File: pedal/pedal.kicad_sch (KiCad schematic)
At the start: 55 parts, among them J1 AudioJack3, J2 AudioJack3, J3 Micro SD, J4 USB_B_Micro, J5 Debug, U1 LP2985-1.8, U2 PCM3060, U3 TPS62172DSG, U4 TL072, U5 STM32H750IBTx, U6 RC4580, Y1 25MHz

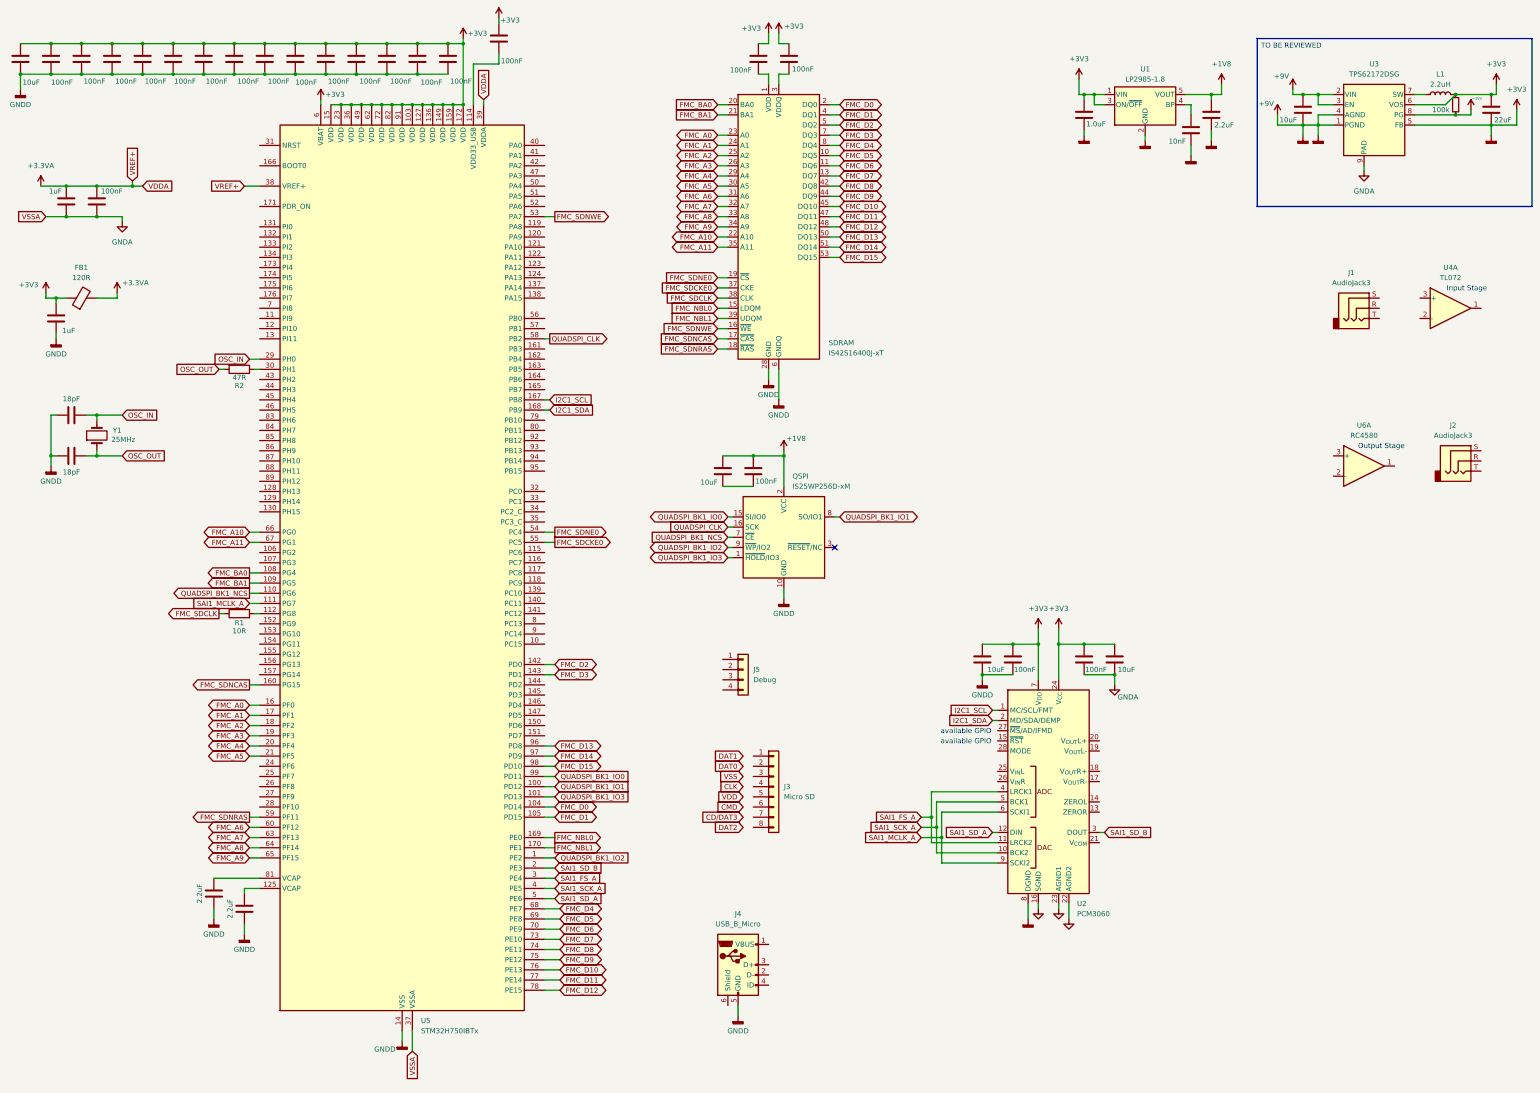
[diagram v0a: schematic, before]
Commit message: update JOURNAL and step down BC
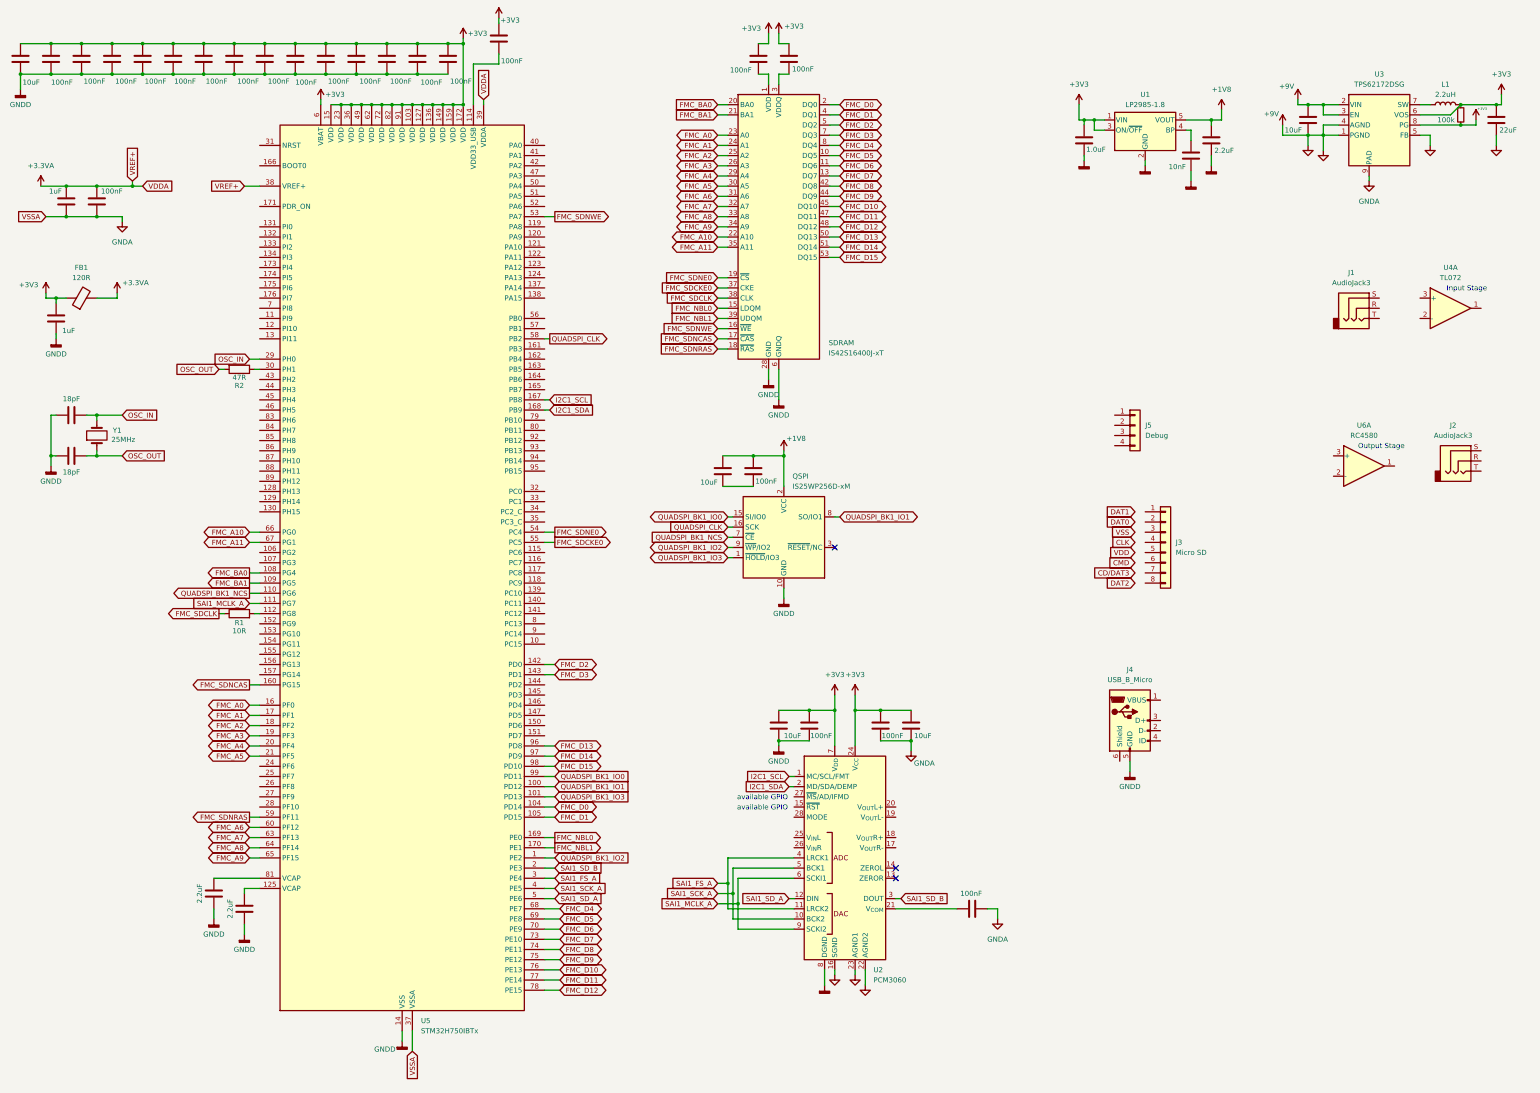
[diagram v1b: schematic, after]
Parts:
- added C37: 100nF, symbol Device:C
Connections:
- net +3V3: no longer C1.1, C10.2, C11.2, C12.2, C13.2, C14.2, C15.2, C16.2, C17.2, C2.1, C21.2, C24.1, C25.1, C26.2, C27.2, C28.2, C29.2, C3.2, C30.1, C30.2, C33.2, C34.2, C4.2, C5.2, C6.2, C7.2, C8.2, C9.2, J4.5 (GND), QSPI.10 (GND), SDRAM.12 (GNDQ), SDRAM.28 (GND), SDRAM.41 (GND), SDRAM.46 (GNDQ), SDRAM.52 (GNDQ), SDRAM.54 (GND), SDRAM.6 (GNDQ), U1.2 (GND), U2.8 (DGND), U3.1 (PGND), U3.2 (VIN), U3.3 (EN), U3.4 (AGND), U3.5 (FB), U5.102 (VSS), U5.113 (VSS), U5.126 (VSS), U5.135 (VSS), U5.14 (VSS), U5.148 (VSS), U5.158 (VSS), U5.22 (VSS), U5.48 (VSS), U5.61 (VSS), U5.71 (VSS), U5.90 (VSS)
- net at U2.21 (V_{COM}): now also C37.1
- net GNDA renamed +9V
- net +9V: now also C29.2, C30.1, C30.2, U3.1 (PGND), U3.2 (VIN), U3.3 (EN), U3.4 (AGND), U3.5 (FB), C37.2
- new net GNDD: C1.1, C10.2, C11.2, C12.2, C13.2, C14.2, C15.2, C16.2, C17.2, C2.1, C21.2, C24.1, C25.1, C26.2, C27.2, C28.2, C3.2, C33.2, C34.2, C4.2, C5.2, C6.2, C7.2, C8.2, C9.2, J4.5 (GND), QSPI.10 (GND), SDRAM.12 (GNDQ), SDRAM.28 (GND), SDRAM.41 (GND), SDRAM.46 (GNDQ), SDRAM.52 (GNDQ), SDRAM.54 (GND), SDRAM.6 (GNDQ), U1.2 (GND), U2.8 (DGND), U5.102 (VSS), U5.113 (VSS), U5.126 (VSS), U5.135 (VSS), U5.14 (VSS), U5.148 (VSS), U5.158 (VSS), U5.22 (VSS), U5.48 (VSS), U5.61 (VSS), U5.71 (VSS), U5.90 (VSS)
- no-connect marks 1 -> 3
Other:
- moved on the sheet: J3, J4, J5, L1, U1, U2, U3
